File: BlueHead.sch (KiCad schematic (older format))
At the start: 38 parts, among them J1 CONN_01X03, J2 CONN_01X06, J3 CONN_01X06, J4 CONN_01X08, J5 CONN_01X06, J6 CONN_01X05, J7 CONN_01X05, J8 CONN_01X05, U1 Bluepill, U2 LM7805

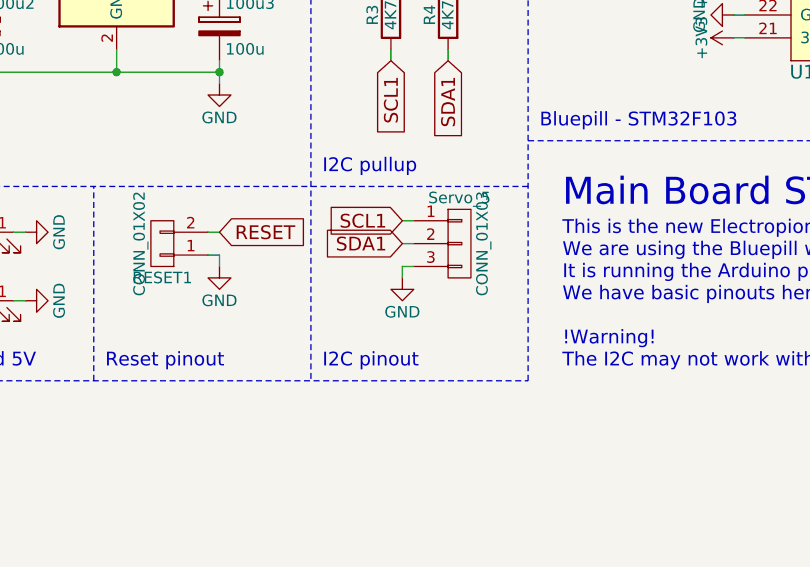
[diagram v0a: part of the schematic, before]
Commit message: Issue resolving
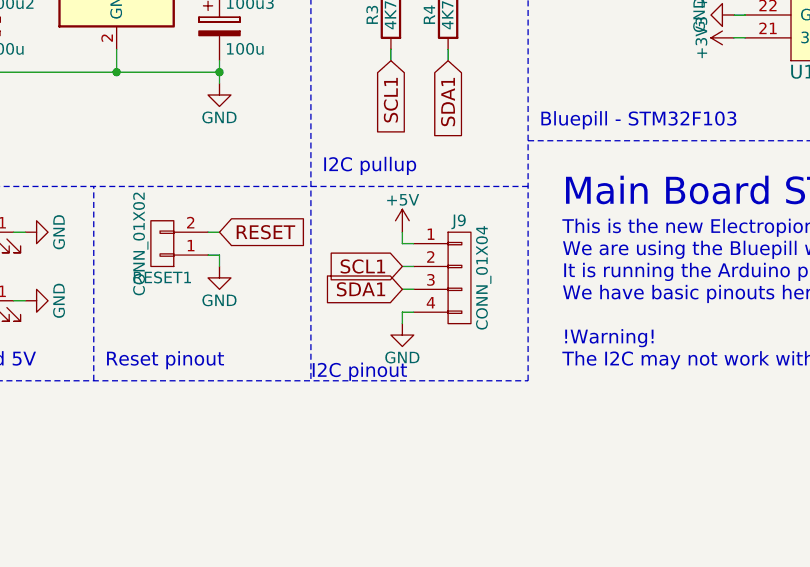
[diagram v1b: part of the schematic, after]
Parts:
- removed Servo_5: CONN_01X03, Pin_Headers:Pin_Header_Straight_1x03_Pitch2.54mm, symbol CONN_01X03
- added J9: CONN_01X04, Pin_Headers:Pin_Header_Straight_1x04_Pitch2.54mm, symbol CONN_01X04
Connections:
- net +5V: now also J9.1 (P1)
- net GND: now also J9.4 (P4)
- net SCL1: now also J9.2 (P2)
- net SDA1: now also J9.3 (P3)
